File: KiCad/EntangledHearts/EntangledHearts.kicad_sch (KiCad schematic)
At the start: 65 parts

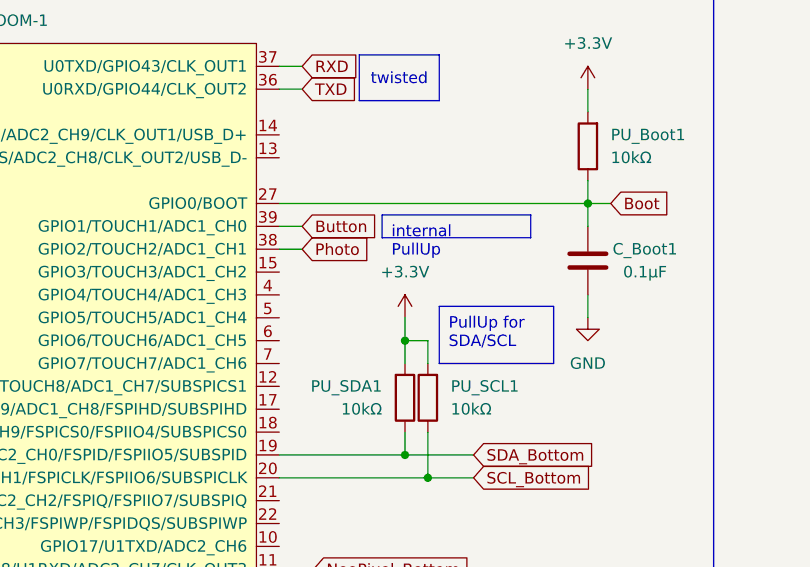
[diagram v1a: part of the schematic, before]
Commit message: ADD: all components connected
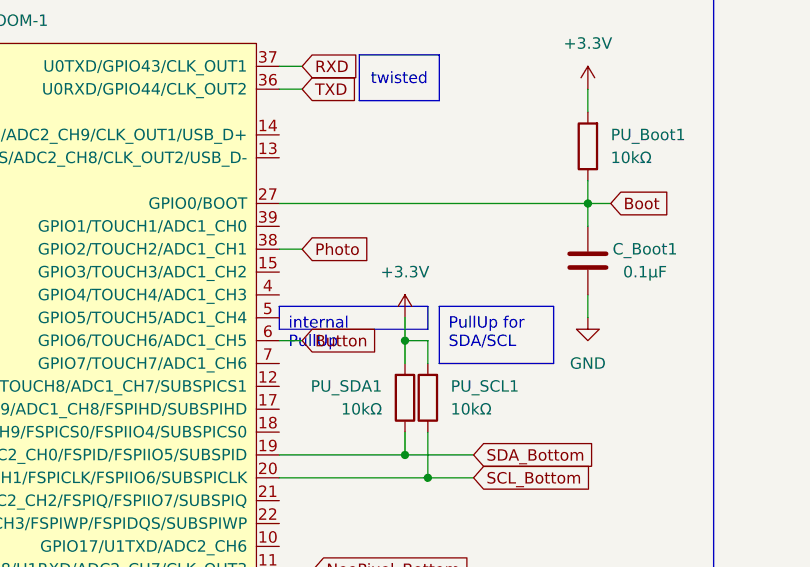
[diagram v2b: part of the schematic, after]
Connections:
- net Button: now also ESP1.6 (GPIO6/TOUCH6/ADC1_CH5); no longer ESP1.39 (GPIO1/TOUCH1/ADC1_CH0)
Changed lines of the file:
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@@
-    (stroke (width 0) (type default))
-  )
-  (wire (pts (xy 260.35 101.6) (xy 262.89 101.6))
     (stroke (width 0) (type default))
   )
@@
   )
   (wire (pts (xy 157.48 238.76) (xy 157.48 236.22))
+    (stroke (width 0) (type default))
+  )
+  (wire (pts (xy 260.35 114.3) (xy 262.89 114.3))
     (stroke (width 0) (type default))
   )
@@
   )
   (text_box "internal PullUp"
-    (at 271.78 100.33 0) (size 16.51 2.54)
+    (at 260.35 110.49 0) (size 16.51 2.54)
     (stroke (width 0) (type default))
     (fill (type none))
@@
     )
   )
-  (global_label "Button" (shape input) (at 262.89 101.6 0) (fields_autoplaced)
-    (effects (font (size 1.27 1.27)) (justify left))
-    (property "Intersheetrefs" "${INTERSHEET_REFS}" (at 272.0436 101.6 0)
-      (effects (font (size 1.27 1.27)) (justify left) hide)
-    )
+  (global_label "Button" (shape input) (at 262.89 114.3 0) (fields_autoplaced)
+    (effects (font (size 1.27 1.27)) (justify left))
+    (property "Intersheetrefs" "${INTERSHEET_REFS}" (at 272.0436 114.3 0)
+      (effects (font (size 1.27 1.27)) (justify left) hide)
+    )
